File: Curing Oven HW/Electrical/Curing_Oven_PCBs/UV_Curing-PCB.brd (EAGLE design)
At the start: 91.1 x 63.5 mm, 18 parts, among them J1 12V_SUP, J2 PINHEADER-5POS-2.54MM, J3 PINHEADER-7POS-2.54MM, J4 UV_SUP, J5 UV_FN, J6 MOTOR, J7 5V_SUP, J8 SPKR, K1 25V, Q1 55V, Q2 55V, Q3 30V 100mA, U1 A000005

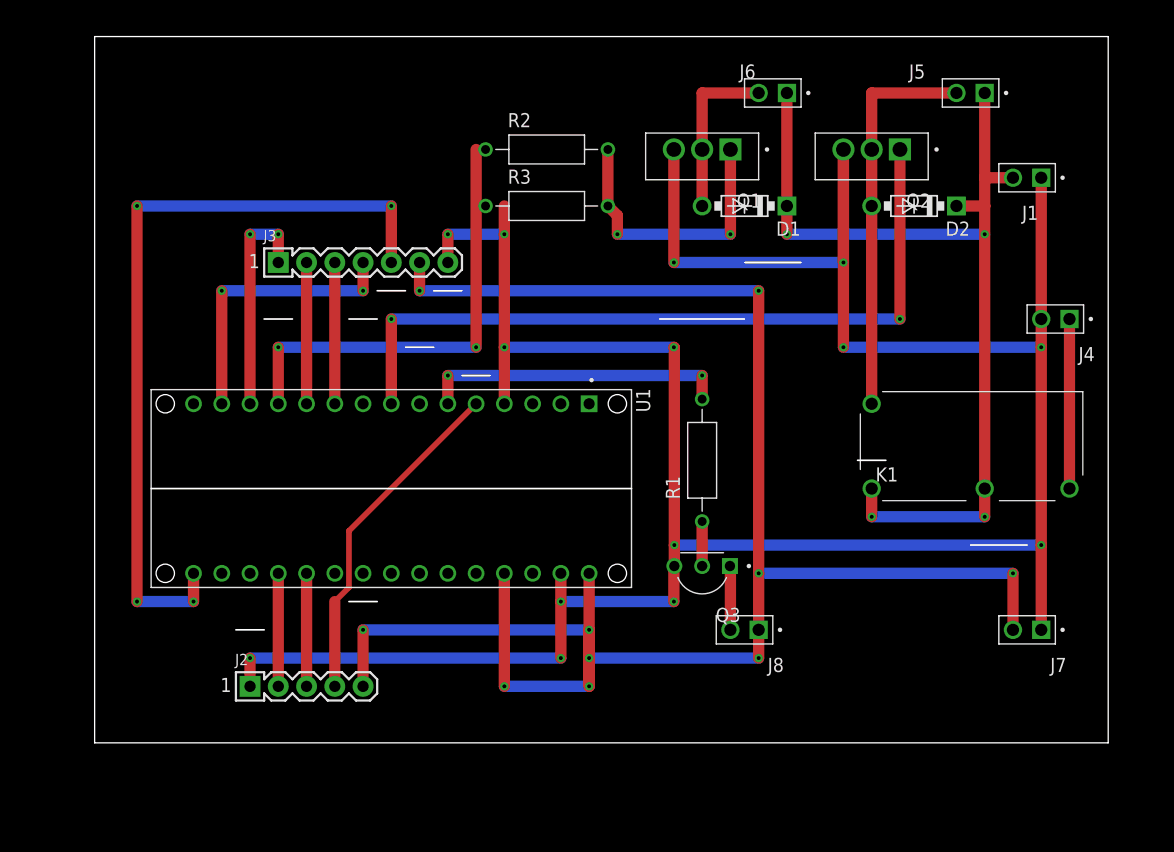
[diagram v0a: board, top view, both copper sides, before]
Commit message: Updated PCB for fab manufacturing
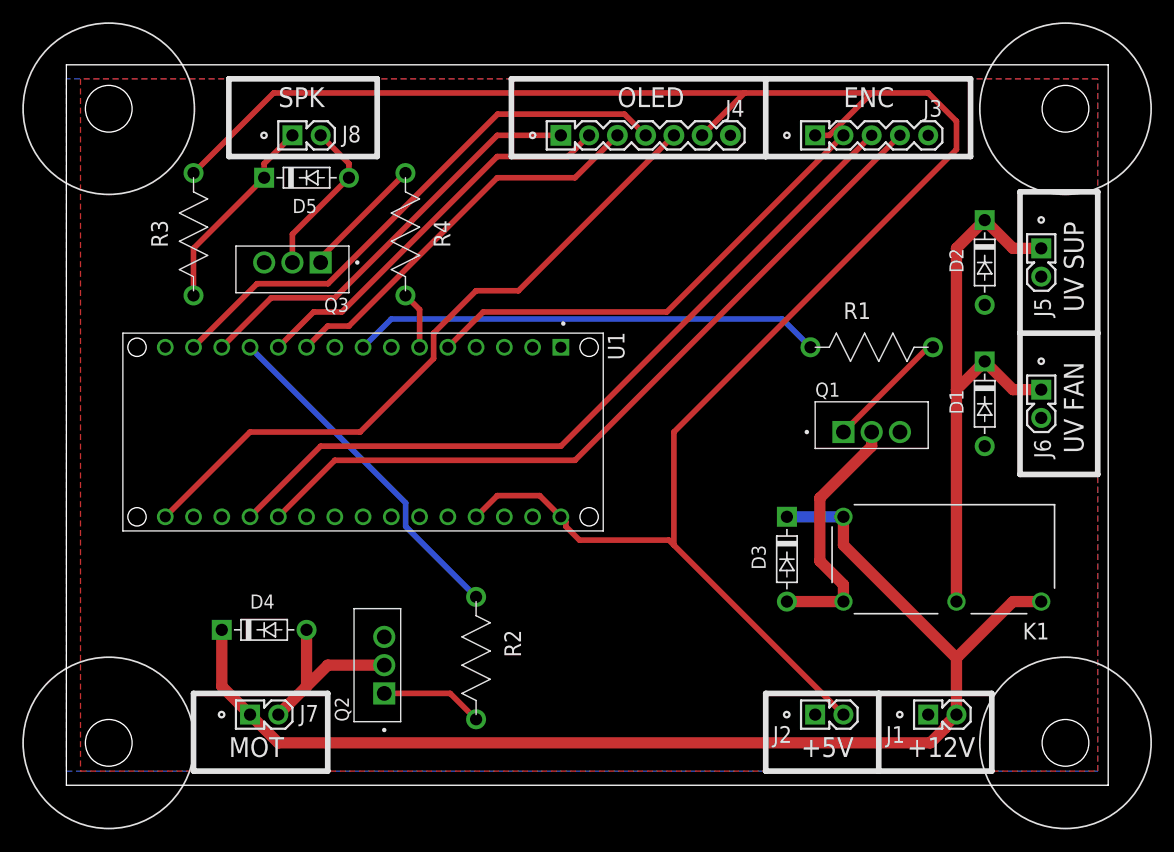
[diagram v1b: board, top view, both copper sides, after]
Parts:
- added D3, D4, D5: 400V, Up3D Active Components:DIOAD520W79L463D238
- added M1, M2, M3, M4: MOUNTING_HOLE, Up3D Misc:M4_NP_MOUNTING_HOLE
- added R4: 1K, Up3D Resistors:RES-THRU
- J1: value 12V_SUP -> PINHEADER-2POS-2.54MM
- J2: value PINHEADER-5POS-2.54MM -> PINHEADER-2POS-2.54MM; device Up3D Misc:254-1X05-PIN -> Up3D Misc:254-1X02-PIN
- J3: value PINHEADER-7POS-2.54MM -> PINHEADER-5POS-2.54MM; device Up3D Misc:254-1X07-PIN -> Up3D Misc:254-1X05-PIN
- J4: value UV_SUP -> PINHEADER-7POS-2.54MM; device Up3D Misc:254-1X02-PIN -> Up3D Misc:254-1X07-PIN
- J5: value UV_FN -> PINHEADER-2POS-2.54MM
- J6: value MOTOR -> PINHEADER-2POS-2.54MM
- J7: value 5V_SUP -> PINHEADER-2POS-2.54MM
- J8: value SPKR -> PINHEADER-2POS-2.54MM
- Q3: value 30V 100mA -> 55V; device Up3D Active Components:BJT-NPN-TO-92-3 -> Up3D Active Components:TO254P1016X419X2286-3
- R1: value 220E -> 1K
- R3: value 10K -> 8E
- moved J7 70.3 mm to (12.7, 2.54), turned to 0 degrees
- moved Q2 63.8 mm to (24.8, 6.99), turned to 90 degrees
- moved J8 60.2 mm to (16.5, 54.6), turned to 0 degrees
- moved J2 50.9 mm to (63.5, 2.54)
- moved J3 49.6 mm to (63.5, 54.6)
- moved J1 49.1 mm to (73.7, 2.54), turned to 0 degrees
- moved J4 47.4 mm to (40.6, 54.6), turned to 0 degrees
- moved Q3 46.2 mm to (16.5, 43.2)
- moved R2 46.2 mm to (33.0, 7.62), turned to 270 degrees
- moved J6 36.0 mm to (83.8, 31.8), turned to 270 degrees
- moved R3 31.9 mm to (7.62, 45.7), turned to 90 degrees
- moved Q1 29.6 mm to (68.6, 27.9), turned to 0 degrees
- moved D1 28.0 mm to (78.7, 30.5), turned to 270 degrees
- moved R1 18.3 mm to (68.6, 35.6), turned to 0 degrees
- moved J5 15.3 mm to (83.8, 44.5), turned to 270 degrees
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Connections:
- net MOTOR_SW renamed MOT_SW
- removed net DI_KEY: J2.4, U1.5
- removed net DI_S1: J2.2, U1.19
- removed net DI_S2: J2.3, U1.20
- removed net SPEAKER_SW: R1.2, U1.6
- removed net UV_SW: Q2.1, U1.8
- new net ENC_KEY: J3.2, U1.5
- new net ENC_S1: J3.4, U1.20
- new net ENC_S2: J3.3, U1.19
- new net LAMP_EN: R1.1, U1.8
- new net N$6: D5.C, J8.01, R3.1
- new net N$9: Q3.1, R4.2
- new net SPK_SW: R4.1, U1.6
- net +12V: now also D3.C, D4.C, J7.01, K1.16, K1.8; no longer D1.C, D2.C, J5.01, J6.01, K1.13, K1.9
- net +5V: now also J2.02, J3.1, J4.6, R3.2; no longer J2.5, J3.6, J7.02, J8.01
- net GND: now also D1.A, D2.A, J2.01, J3.5, J4.7, J5.02, J6.02; no longer J2.1, J3.7, J4.02, J7.01, R3.1
- net N$1: now also Q1.1, R1.2; no longer D1.A, J6.02, Q1.2
- net N$2: now also D1.C, D2.C, J5.01, J6.01, K1.13; no longer J4.01, K1.16
- net N$3: now also D3.A, K1.9, Q1.2; no longer Q1.1, R2.2, R3.2
- net N$4: now also Q2.1, R2.2; no longer D2.A, J5.02, K1.8, Q2.2
- net N$5: now also D4.A, J7.02, Q2.2; no longer J8.02, Q3.1
- net N$7: now also D5.A, J8.02; no longer R1.1
- net OLED_CLK: now also J4.5; no longer J3.5
- net OLED_CS: now also J4.1; no longer J3.1
- net OLED_DC: now also J4.2; no longer J3.2
- net OLED_MOSI: now also J4.4; no longer J3.4
- net OLED_RST: now also J4.3; no longer J3.3
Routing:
- net GND: track 256.5 -> 0.00 mm, vias 14 -> 0
- net ENC_S2: track 0.00 -> 70.1 mm
- net ENC_S1: track 0.00 -> 70.1 mm
- net UV_SW: track 68.6 -> 0.00 mm, vias 2 -> 0
- net ENC_KEY: track 0.00 -> 43.5 mm
- net LAMP_EN: track 0.00 -> 42.3 mm
- net N$2: track 15.2 -> 51.2 mm
- net DI_KEY: track 30.7 -> 0.00 mm
- net SPEAKER_SW: track 27.5 -> 0.00 mm, vias 2 -> 0
- net N$4: track 35.6 -> 9.22 mm
- net +12V: track 86.4 -> 111.2 mm, vias 4 -> 0
- net OLED_MOSI: track 25.4 -> 50.1 mm, vias 2 -> 0
- net OLED_RST: track 12.7 -> 35.8 mm
- net OLED_DC: track 12.7 -> 35.8 mm
- net N$6: track 0.00 -> 18.1 mm
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- added copper zone on layer 1, net GND
- added copper zone on layer 16, net GND
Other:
- board size 91.1 x 63.5 mm -> 93.7 x 64.8 mm
- board text added: "+12V"
- board text added: "+5V"
- board text added: "ENC"
- board text added: "MOT"
- board text added: "OLED"
- board text added: "SPK"
- board text added: "UV FAN"
- board text added: "UV SUP"
